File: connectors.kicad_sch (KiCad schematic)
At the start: 16 parts

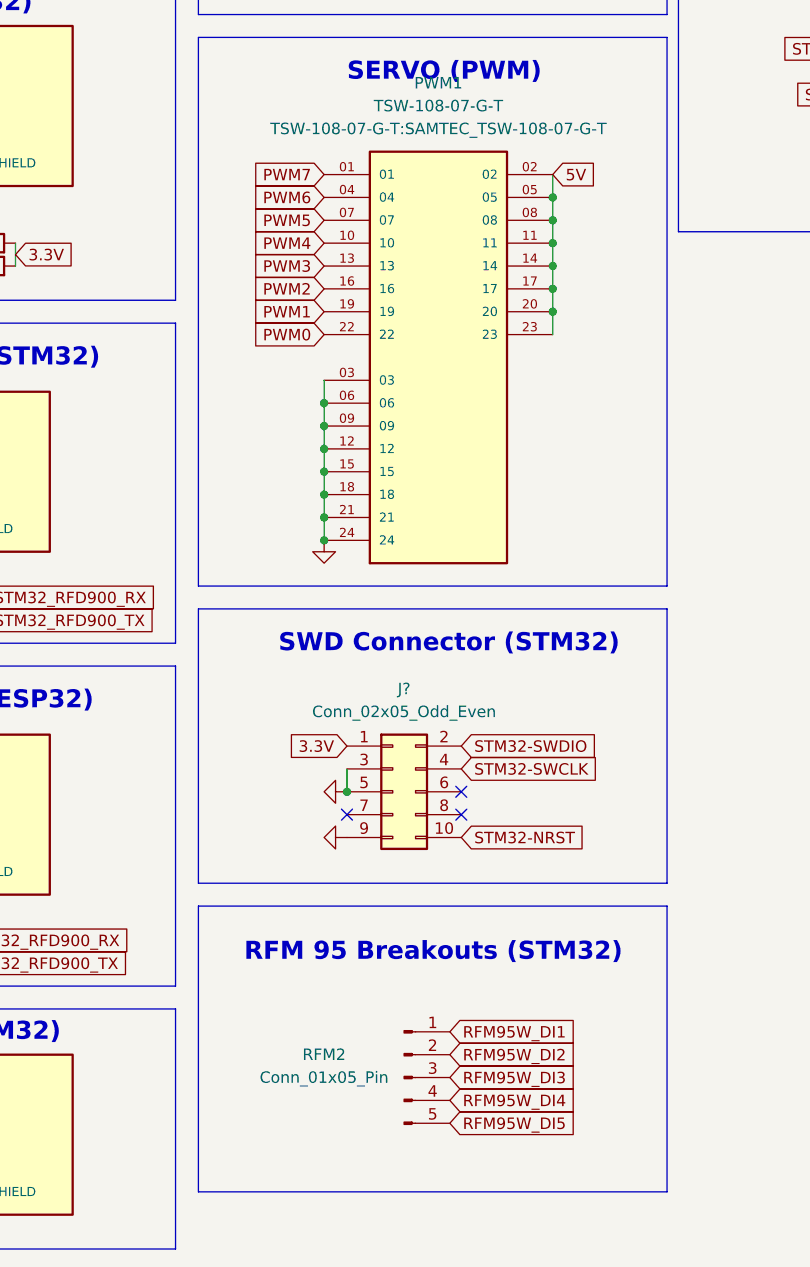
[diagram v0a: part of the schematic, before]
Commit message: started routing
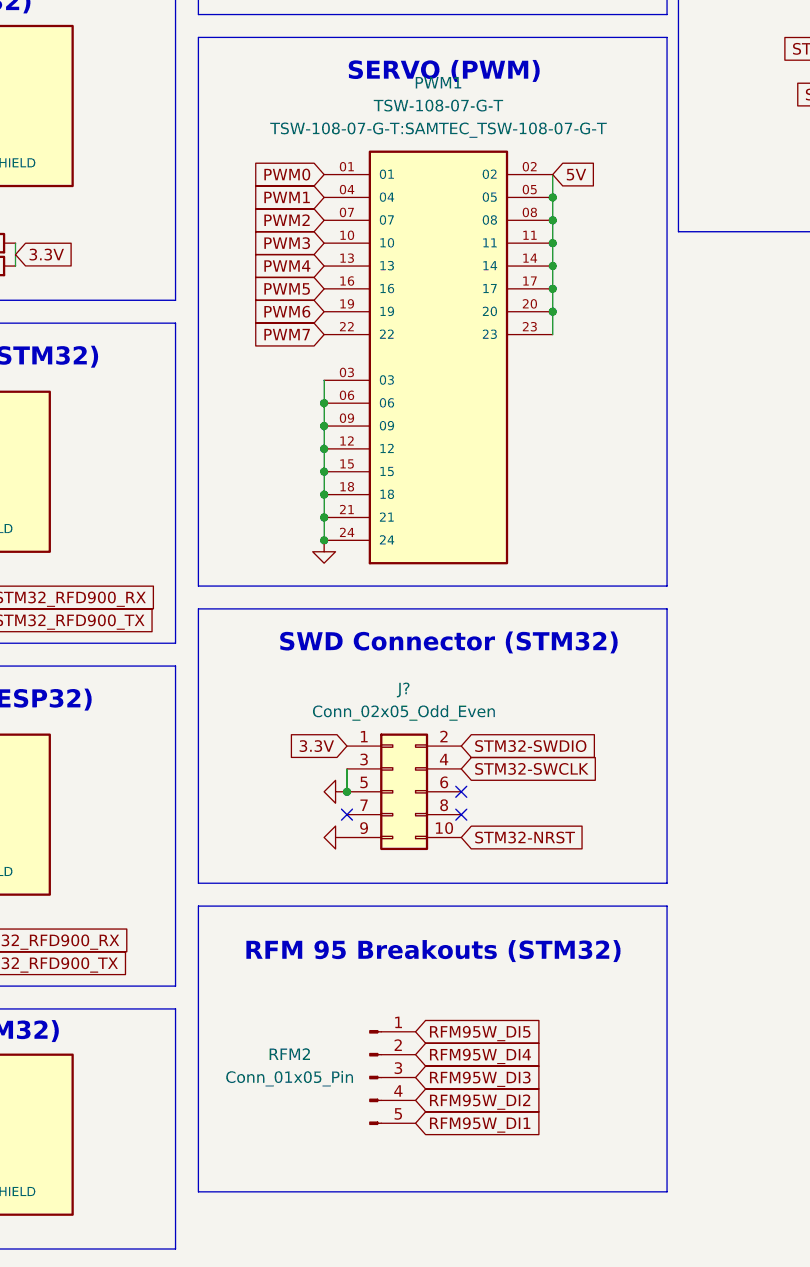
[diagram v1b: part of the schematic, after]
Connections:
- net PWM0: now also PWM1.01; no longer PWM1.22
- net PWM1: now also PWM1.04; no longer PWM1.19
- net PWM2: now also PWM1.07; no longer PWM1.16
- net PWM3: now also PWM1.10; no longer PWM1.13
- net PWM4: now also PWM1.13; no longer PWM1.10
- net PWM5: now also PWM1.16; no longer PWM1.07
- net PWM6: now also PWM1.19; no longer PWM1.04
- net PWM7: now also PWM1.22; no longer PWM1.01
- net RFM95W_DI1: now also RFM2.5 (Pin_5); no longer RFM2.1 (Pin_1)
- net RFM95W_DI2: now also RFM2.4 (Pin_4); no longer RFM2.2 (Pin_2)
- net RFM95W_DI4: now also RFM2.2 (Pin_2); no longer RFM2.4 (Pin_4)
- net RFM95W_DI5: now also RFM2.1 (Pin_1); no longer RFM2.5 (Pin_5)
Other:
- moved on the sheet: RFM2

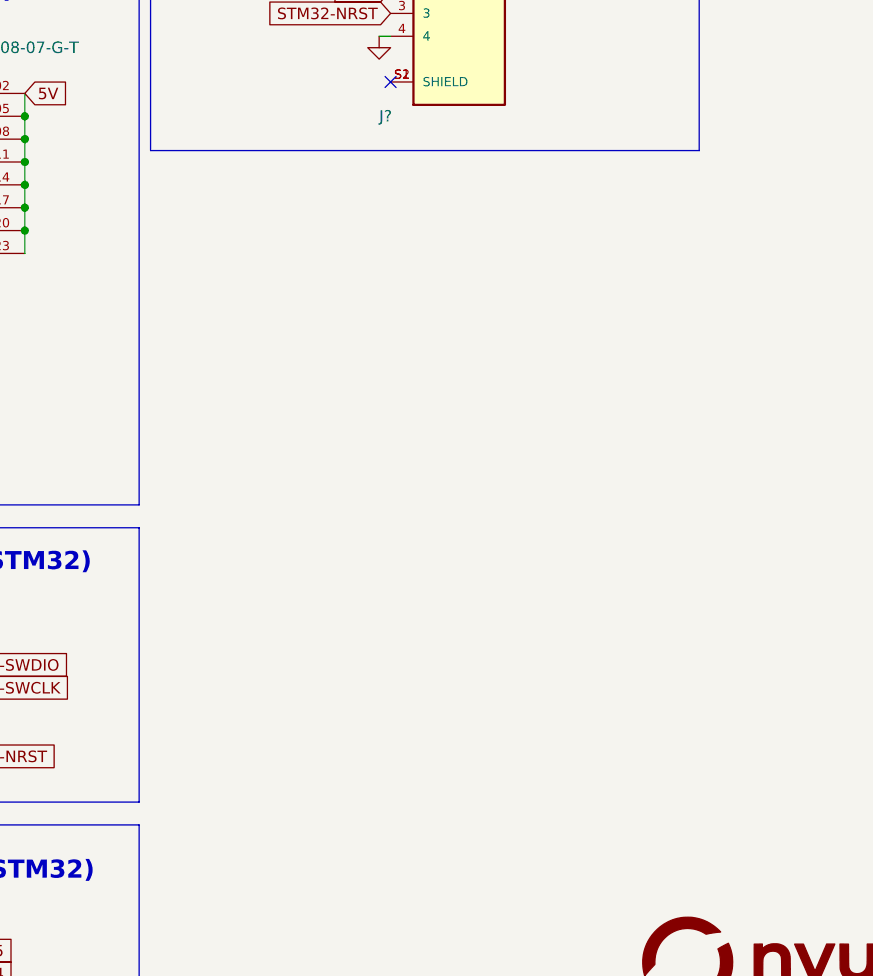
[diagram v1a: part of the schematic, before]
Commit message: more routing
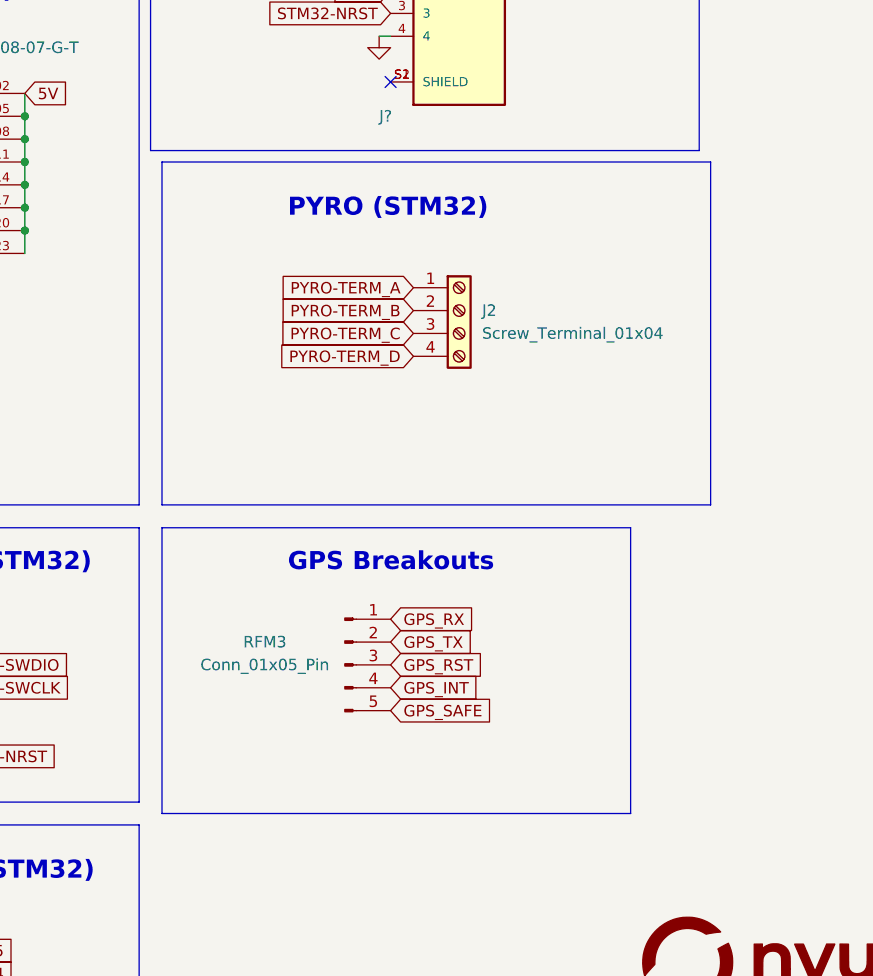
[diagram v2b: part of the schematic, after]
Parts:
- added J2: Screw_Terminal_01x04, TerminalBlock_TE-Connectivity:TerminalBlock_TE_282834-4_1x04_P2.54mm_Horizontal, symbol Connector:Screw_Terminal_01x04
- added RFM3: Conn_01x05_Pin, Connector_PinHeader_1.27mm:PinHeader_1x05_P1.27mm_Vertical, symbol Connector:Conn_01x05_Pin
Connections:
- new net GPS_INT: RFM3.4 (Pin_4)
- new net GPS_RST: RFM3.3 (Pin_3)
- new net GPS_RX: RFM3.1 (Pin_1)
- new net GPS_SAFE: RFM3.5 (Pin_5)
- new net GPS_TX: RFM3.2 (Pin_2)
- new net PYRO-TERM_A: J2.1 (Pin_1)
- new net PYRO-TERM_B: J2.2 (Pin_2)
- new net PYRO-TERM_C: J2.3 (Pin_3)
- new net PYRO-TERM_D: J2.4 (Pin_4)
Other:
- note added: "GPS Breakouts"
- note added: "PYRO (STM32)"
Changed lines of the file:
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@@
+    (fill (type none))
+  )
+  (rectangle (start 124.46 124.46) (end 176.53 156.21)
+    (stroke (width 0) (type default))
     (fill (type none))
   )
@@
     (fill (type none))
   )
+  (rectangle (start 124.46 83.82) (end 185.42 121.92)
+    (stroke (width 0) (type default))
+    (fill (type none))
+  )
   (rectangle (start 69.85 60.96) (end 121.92 121.92)
     (stroke (width 0) (type default))
@@
     (effects (font (size 2 2) (thickness 0.8) bold) (justify left bottom))
   )
+  (text "PYRO (STM32)" (at 138.43 90.17 0)
+    (effects (font (size 2 2) (thickness 0.8) bold) (justify left bottom))
+  )
   (text "SWD Connector (STM32)" (at 78.74 129.54 0)
     (effects (font (size 2 2) (thickness 0.8) bold) (justify left bottom))
@@
     (effects (font (size 1.27 1.27) bold) (justify left bottom))
   )
+  (text "GPS Breakouts\n" (at 138.43 129.54 0)
+    (effects (font (size 2 2) (thickness 0.8) bold) (justify left bottom))
+  )
   (text "RFD UART 1 (STM32)" (at 26.67 97.79 0)
     (effects (font (size 2 2) (thickness 0.8) bold) (justify left bottom))
@@
     )
   )
+  (global_label "GPS_RX" (shape input) (at 149.86 134.62 0) (fields_autoplaced)
+    (effects (font (size 1.27 1.27)) (justify left))
+    (property "Intersheetrefs" "${INTERSHEET_REFS}" (at 160.0418 134.62 0)
+      (effects (font (size 1.27 1.27)) (justify left) hide)
+    )
+  )
   (global_label "ESP32-I2C1_SCL" (shape input) (at 41.91 86.36 180) (fields_autoplaced)
     (effects (font (size 1.27 1.27)) (justify right))
@@
     )
   )
+  (global_label "GPS_TX" (shape input) (at 149.86 137.16 0) (fields_autoplaced)
+    (effects (font (size 1.27 1.27)) (justify left))
+    (property "Intersheetrefs" "${INTERSHEET_REFS}" (at 159.7394 137.16 0)
+      (effects (font (size 1.27 1.27)) (justify left) hide)
+    )
+  )
   (global_label "INA219_SCL" (shape input) (at 251.46 53.34 0) (fields_autoplaced)
     (effects (font (size 1.27 1.27)) (justify left))
@@
     )
   )
+  (global_label "GPS_SAFE" (shape input) (at 149.86 144.78 0) (fields_autoplaced)
+    (effects (font (size 1.27 1.27)) (justify left))
+    (property "Intersheetrefs" "${INTERSHEET_REFS}" (at 162.098 144.78 0)
+      (effects (font (size 1.27 1.27)) (justify left) hide)
+    )
+  )
+  (global_label "PYRO-TERM_C" (shape input) (at 152.4 102.87 180) (fields_autoplaced)
+    (effects (font (size 1.27 1.27)) (justify right))
+    (property "Intersheetrefs" "${INTERSHEET_REFS}" (at 135.8077 102.87 0)
+      (effects (font (size 1.27 1.27)) (justify right) hide)
+    )
+  )
   (global_label "ESP32_RFD900_TX" (shape input) (at 40.64 148.59 180) (fields_autoplaced)
     (effects (font (size 1.27 1.27)) (justify right))
@@
     )
   )
+  (global_label "PYRO-TERM_A" (shape input) (at 152.4 97.79 180) (fields_autoplaced)
+    (effects (font (size 1.27 1.27)) (justify right))
+    (property "Intersheetrefs" "${INTERSHEET_REFS}" (at 135.9891 97.79 0)
+      (effects (font (size 1.27 1.27)) (justify right) hide)
+    )
+  )
   (global_label "H3LIS331DL_SDO" (shape input) (at 255.27 106.68 0) (fields_autoplaced)
     (effects (font (size 1.27 1.27)) (justify left))
@@
     )
   )
+  (global_label "PYRO-TERM_B" (shape input) (at 152.4 100.33 180) (fields_autoplaced)
+    (effects (font (size 1.27 1.27)) (justify right))
+    (property "Intersheetrefs" "${INTERSHEET_REFS}" (at 135.8077 100.33 0)
+      (effects (font (size 1.27 1.27)) (justify right) hide)
+    )
+  )
   (global_label "SD_CS" (shape input) (at 255.27 135.89 0) (fields_autoplaced)
     (effects (font (size 1.27 1.27)) (justify left))
@@
     )
   )
+  (global_label "GPS_INT" (shape input) (at 149.86 142.24 0) (fields_autoplaced)
+    (effects (font (size 1.27 1.27)) (justify left))
+    (property "Intersheetrefs" "${INTERSHEET_REFS}" (at 160.4652 142.24 0)
+      (effects (font (size 1.27 1.27)) (justify left) hide)
+    )
+  )
   (global_label "STM32-SPI2_CS0" (shape input) (at 250.19 124.46 180) (fields_autoplaced)
     (effects (font (size 1.27 1.27)) (justify right))
@@
     )
   )
+  (global_label "PYRO-TERM_D" (shape input) (at 152.4 105.41 180) (fields_autoplaced)
+    (effects (font (size 1.27 1.27)) (justify right))
+    (property "Intersheetrefs" "${INTERSHEET_REFS}" (at 135.8077 105.41 0)
+      (effects (font (size 1.27 1.27)) (justify right) hide)
+    )
+  )
   (global_label "5V" (shape input) (at 40.64 105.41 180) (fields_autoplaced)
     (effects (font (size 1.27 1.27)) (justify right))
@@
     (property "Intersheetrefs" "${INTERSHEET_REFS}" (at 233.1745 158.75 0)
       (effects (font (size 1.27 1.27)) (justify right) hide)
+    )
+  )
+  (global_label "GPS_RST" (shape input) (at 149.86 139.7 0) (fields_autoplaced)
+    (effects (font (size 1.27 1.27)) (justify left))
+    (property "Intersheetrefs" "${INTERSHEET_REFS}" (at 161.0094 139.7 0)
+      (effects (font (size 1.27 1.27)) (justify left) hide)
     )
   )
@@
         (path "/e12346fa-509d-4de9-8ab1-dced307292db/7d58c90a-6730-4b63-ae17-c9d1fe4b2f54"
           (reference "#PWR0166") (unit 1)
+        )
+      )
+    )
+  )
+  (symbol (lib_id "Connector:Conn_01x05_Pin") (at 144.78 139.7 0) (unit 1)
+    (in_bom yes) (on_board yes) (dnp no)
+    (property "Reference" "RFM3" (at 135.89 137.16 0)
+      (effects (font (size 1.27 1.27)))
+    )
+    (property "Value" "Conn_01x05_Pin" (at 135.89 139.7 0)
+      (effects (font (size 1.27 1.27)))
+    )
+    (property "Footprint" "Connector_PinHeader_1.27mm:PinHeader_1x05_P1.27mm_Vertical" (at 144.78 139.7 0)
+      (effects (font (size 1.27 1.27)) hide)
+    )
+    (property "Datasheet" "~" (at 144.78 139.7 0)
+      (effects (font (size 1.27 1.27)) hide)
+    )
+    (pin "1")
+    (pin "2")
+    (pin "3")
+    (pin "4")
+    (pin "5")
+    (instances
+      (project "aether"
+        (path "/e12346fa-509d-4de9-8ab1-dced307292db/7d58c90a-6730-4b63-ae17-c9d1fe4b2f54"
+          (reference "RFM3") (unit 1)
         )
       )
@@
         )
       )
+    )
+  )
+  (symbol (lib_id "Connector:Screw_Terminal_01x04") (at 157.48 100.33 0) (unit 1)
+    (in_bom yes) (on_board yes) (dnp no) (fields_autoplaced)
+    (property "Reference" "J2" (at 160.02 100.33 0)
+      (effects (font (size 1.27 1.27)) (justify left))
+    )
+    (property "Value" "Screw_Terminal_01x04" (at 160.02 102.87 0)
+      (effects (font (size 1.27 1.27)) (justify left))
+    )
+    (property "Footprint" "TerminalBlock_TE-Connectivity:TerminalBlock_TE_282834-4_1x04_P2.54mm_Horizontal" (at 157.48 100.33 0)
+      (effects (font (size 1.27 1.27)) hide)
+    )
+    (property "Datasheet" "~" (at 157.48 100.33 0)
+      (effects (font (size 1.27 1.27)) hide)
+    )
+    (pin "1")
+    (pin "2")
+    (pin "3")
+    (pin "4")
+    (instances
+      (project "aether"
+        (path "/e12346fa-509d-4de9-8ab1-dced307292db/7d58c90a-6730-4b63-ae17-c9d1fe4b2f54"
+          (reference "J2") (unit 1)
+        )
+      )

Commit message: significant amount of routing done
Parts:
- R? (x2): footprint Resistor_SMD:R_0603_1608Metric -> Resistor_SMD:R_0402_1005Metric
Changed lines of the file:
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@@
       (effects (font (size 1.27 1.27)))
     )
-    (property "Footprint" "Resistor_SMD:R_0603_1608Metric" (at 45.72 85.598 90)
+    (property "Footprint" "Resistor_SMD:R_0402_1005Metric" (at 45.72 85.598 90)
       (effects (font (size 1.27 1.27)) hide)
     )
@@
       (effects (font (size 1.27 1.27)))
     )
-    (property "Footprint" "Resistor_SMD:R_0603_1608Metric" (at 45.72 88.138 90)
-      (effects (font (size 1.27 1.27)) hide)
-    )
+    (property "Footprint" "Resistor_SMD:R_0402_1005Metric" (at 45.72 88.138 90)
+      (effects (font (size 1.27 1.27)) hide)
+    )
